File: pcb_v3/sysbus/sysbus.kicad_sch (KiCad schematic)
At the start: 66 parts, among them J1 bus ula 2, J11 bus clu 2, J12 bus clu 3, J19 9V 1A, J2 bus ula 1, J20 VOLTS, J21 AMPS, J22 bus ioc 2, J23 bus ioc 1, J24 bus ioc 3, J26 bus clock, J3 bus rf16 1, J4 bus rf16 2, J5 bus mem 1, J6 bus mem 2, J7 bus clu 1, Q1 BC548, Q2 BC548, SW1 RESET, U1 MC14495P, U10 MC14495P, U11 ADDR N1, U12 DATA N0, U13 MC14495P, U14 RDADDR_LOW, U17 RDADDR_HIGH, U2 ADDR N3, U21 MC14495P, U22 WRADDR_HIGH, U23 WRADDR_LOW, U3 MC14495P, U31 MC14495P, U34 LM7805, U4 ADDR N2, U5 NE555P, U6 MC14495P, U7 DATA N1, U8 MC14495P, U9 ADDR N0

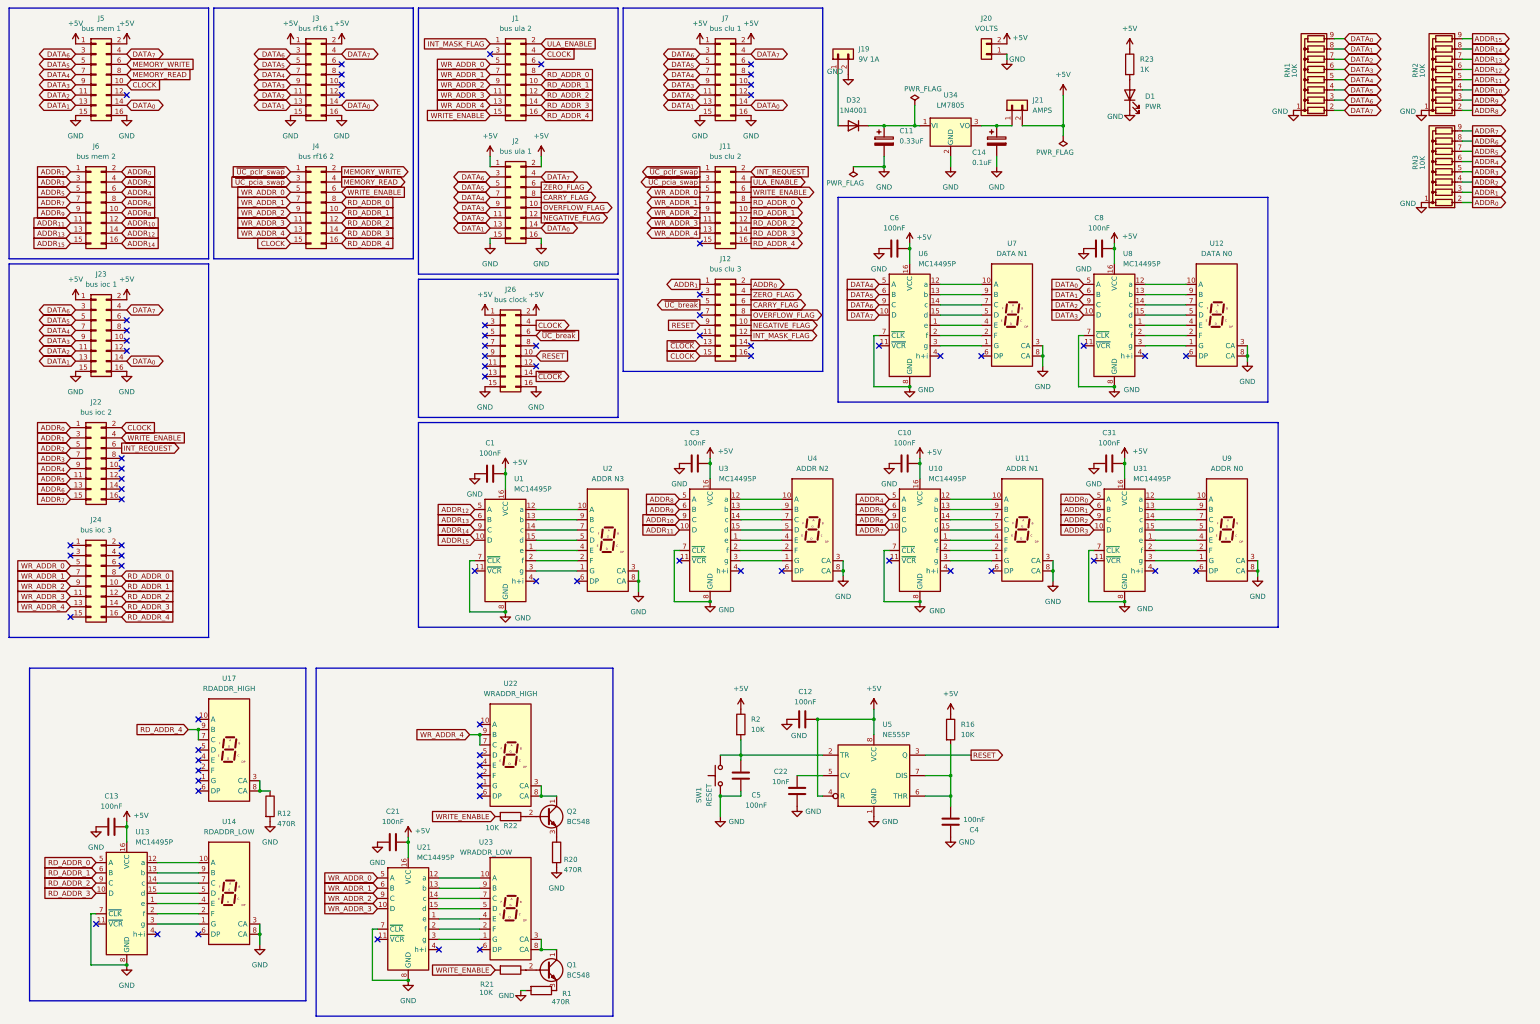
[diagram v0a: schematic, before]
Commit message: refazendo o layout do pcb
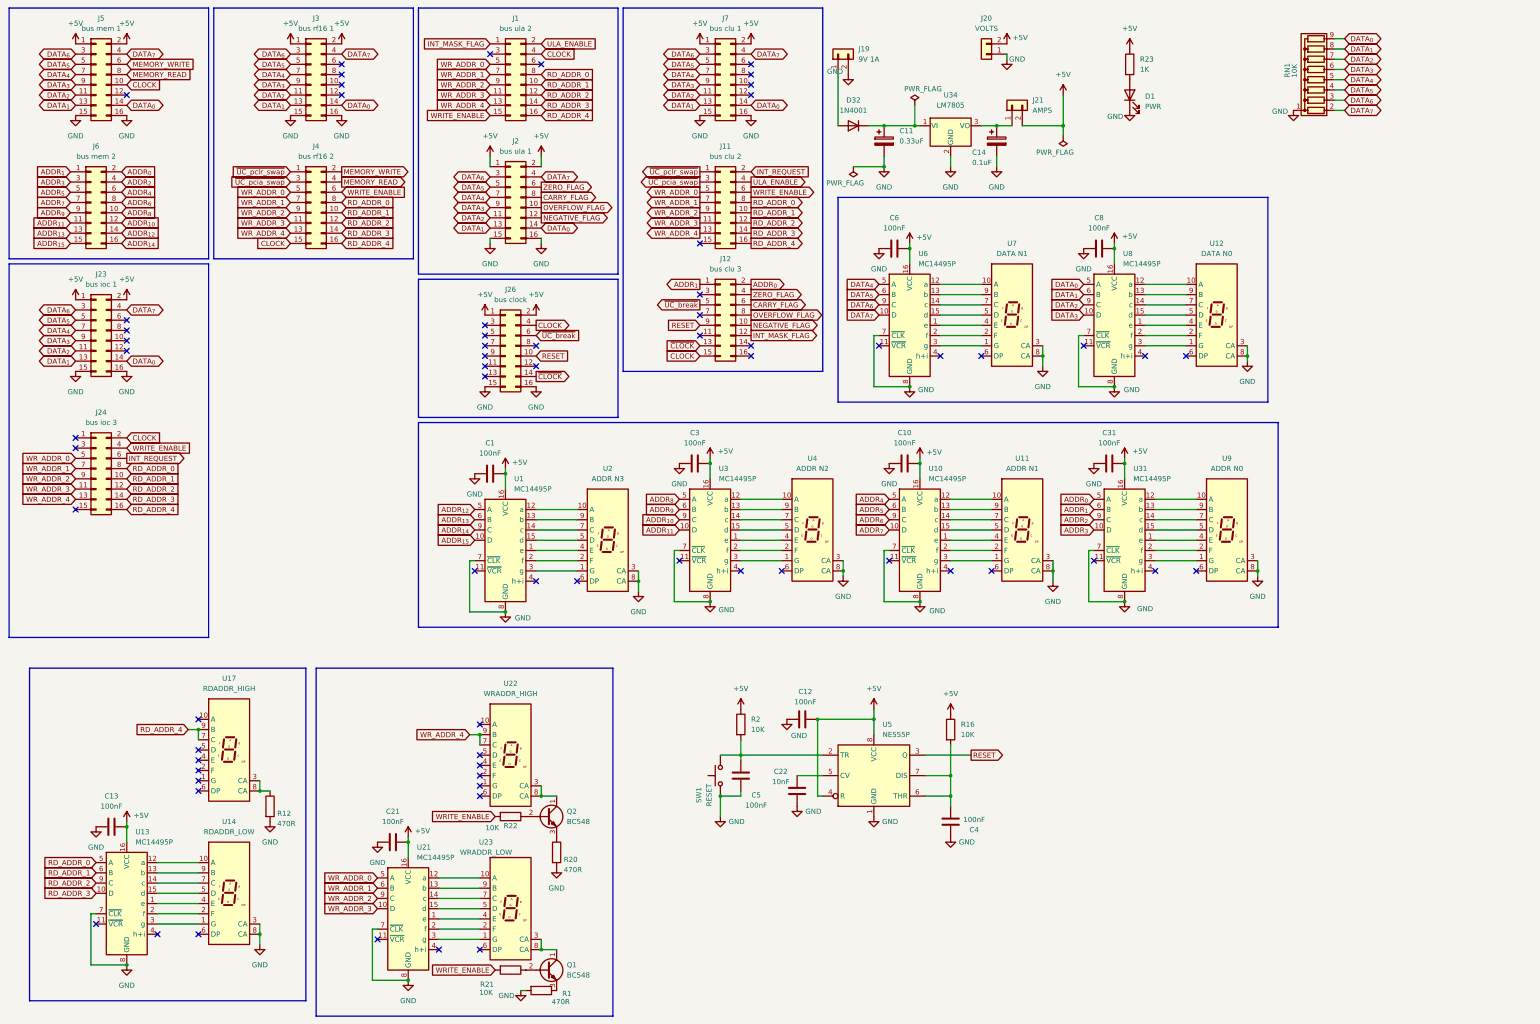
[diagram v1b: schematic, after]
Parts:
- removed J22: bus ioc 2, edge_connector:conector 02x08, symbol Connector_Generic:Conn_02x08_Odd_Even
- removed RN2, RN3: 10K, Resistor_THT:R_Array_SIP9, symbol Device:R_Network08
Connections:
- net CLOCK: now also J24.2 (Pin_2)
- net INT_REQUEST: now also J24.6 (Pin_6)
- net WRITE_ENABLE: now also J24.4 (Pin_4)
- no-connect marks 76 -> 68
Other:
- moved on the sheet: J24
